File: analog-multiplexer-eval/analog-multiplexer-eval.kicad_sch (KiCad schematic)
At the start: 1 part, among them U1 4051

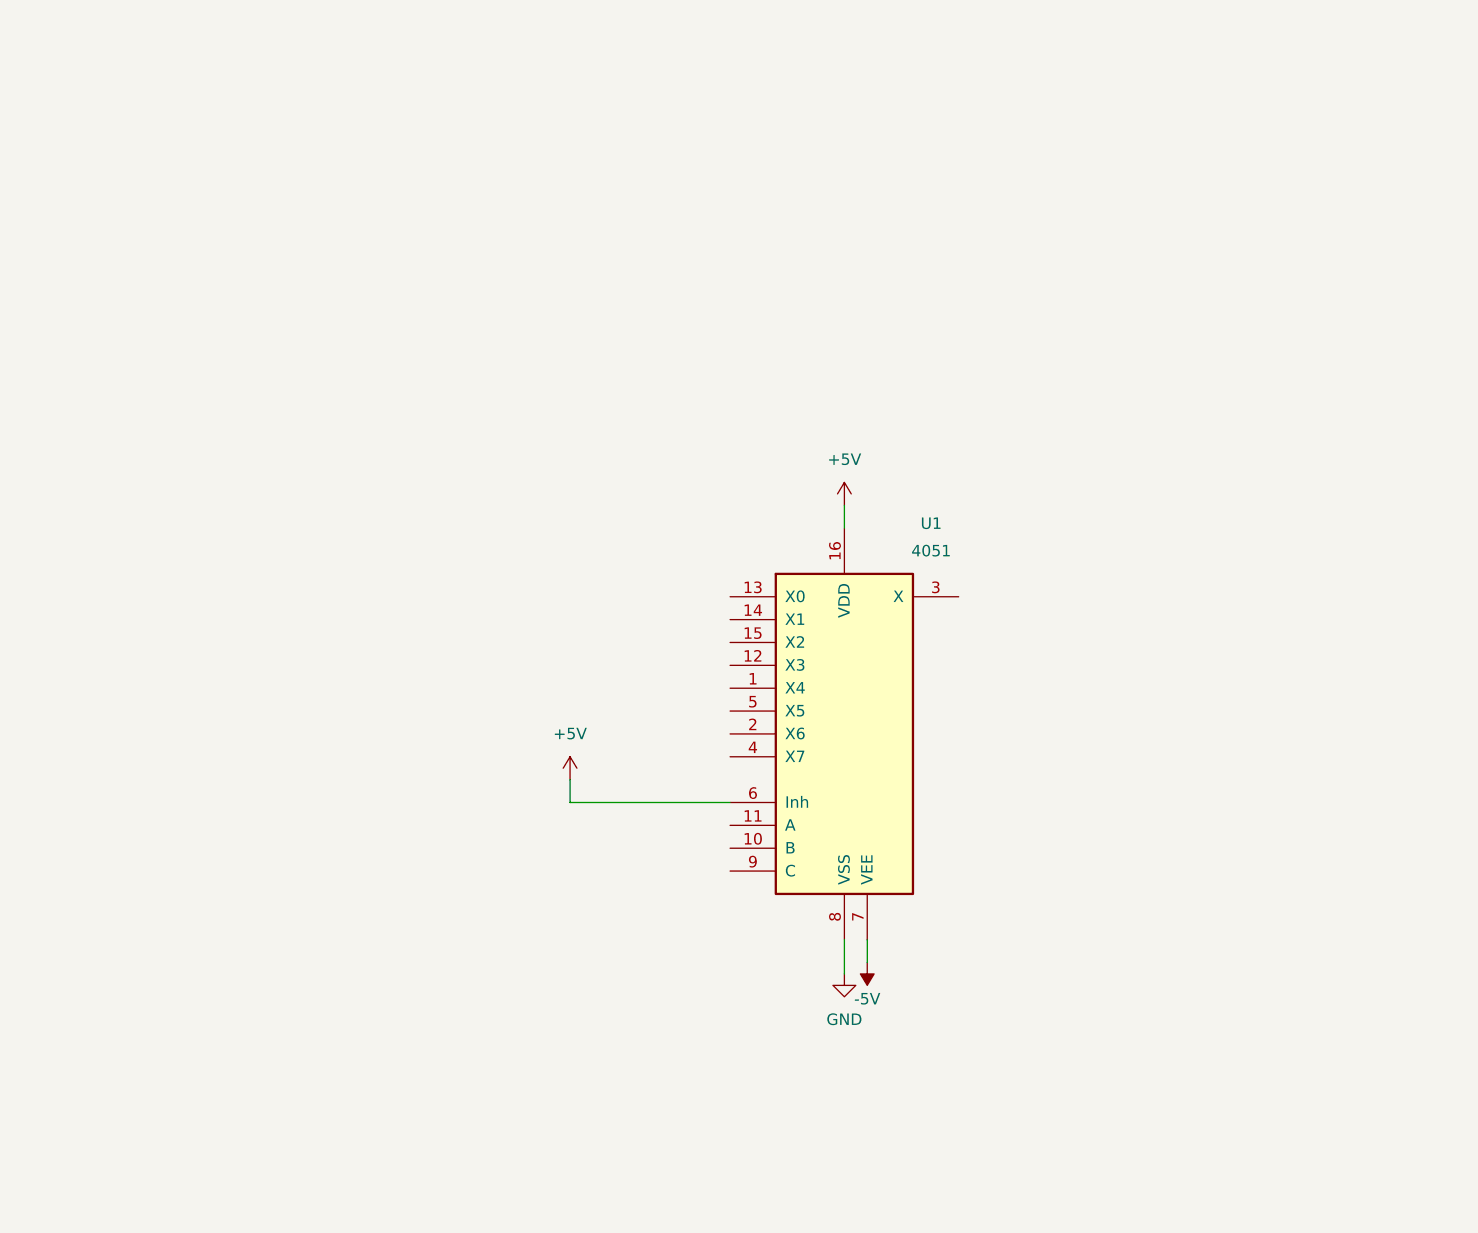
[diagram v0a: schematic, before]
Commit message: dvgsdgsd
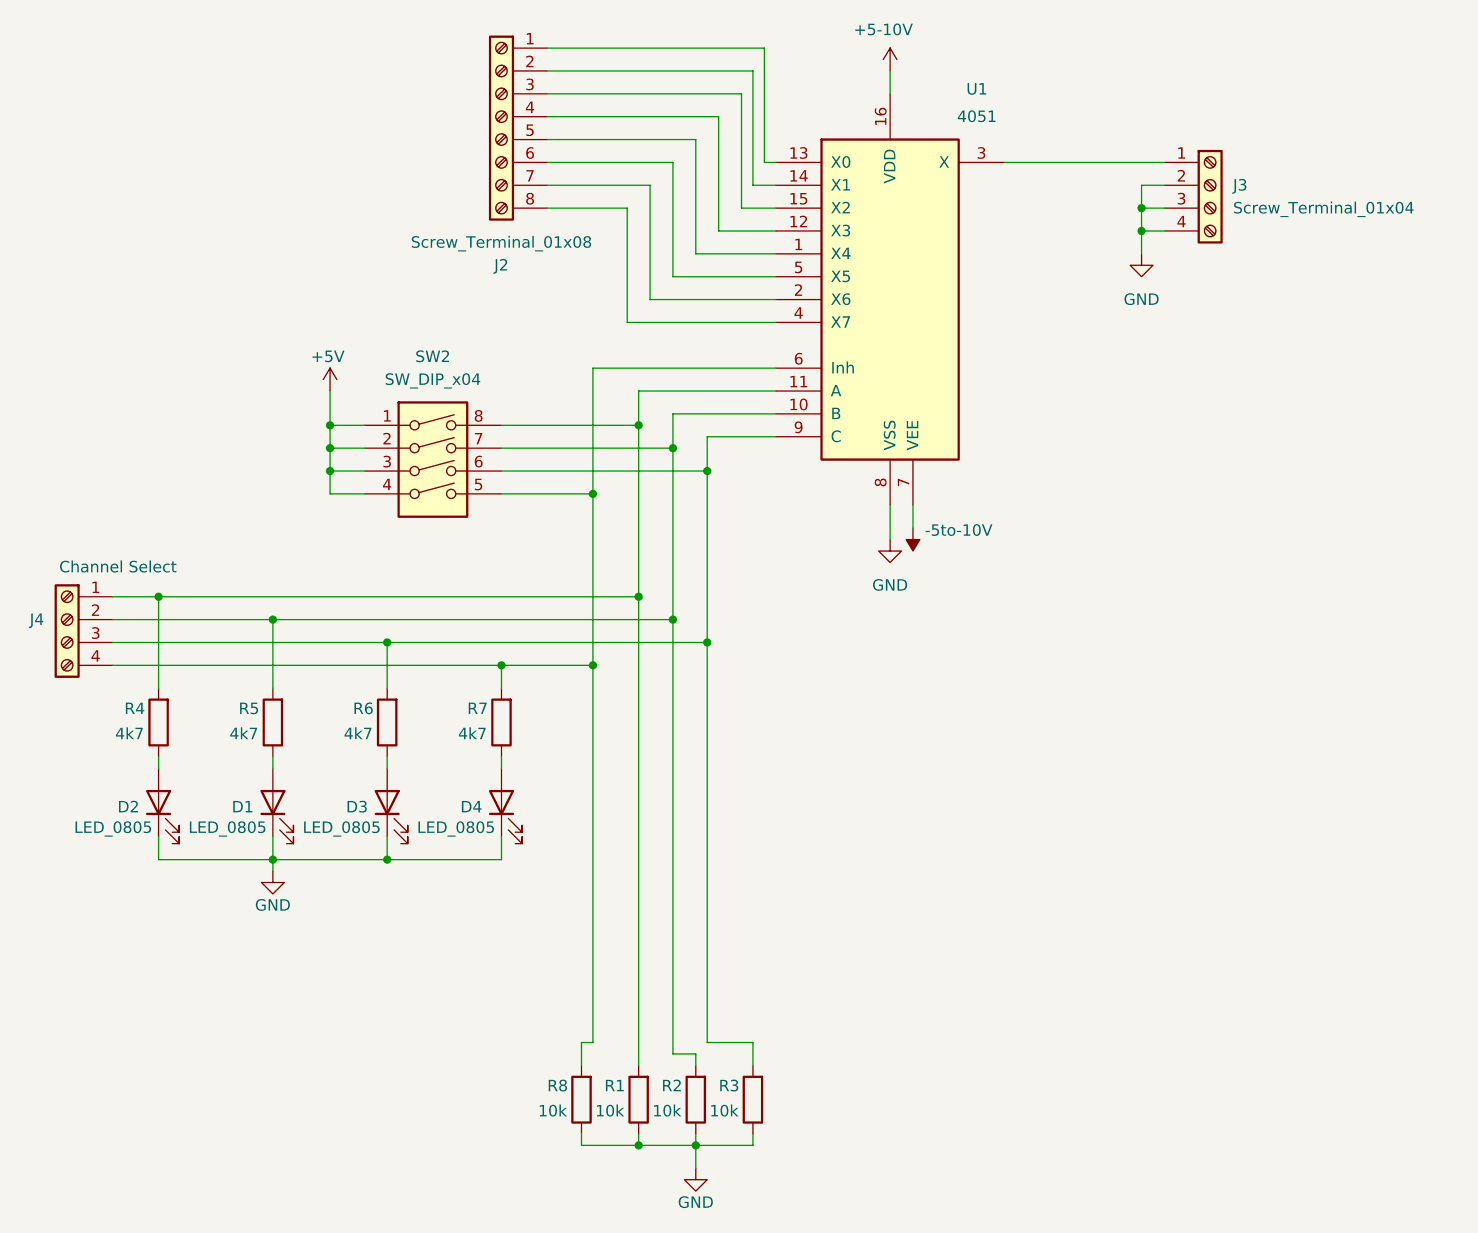
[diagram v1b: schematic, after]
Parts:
- added D1, D2, D3, D4: LED_0805, 000_Diodes_Immo:LED_0805_2012_Kawaii, symbol 000_Diodes_Immo:LED_0805_kawaii
- added J2: Screw_Terminal_01x08, symbol Connector:Screw_Terminal_01x08
- added J3: Screw_Terminal_01x04, symbol Connector:Screw_Terminal_01x04
- added J4: Channel Select, symbol Connector:Screw_Terminal_01x04
- added R1, R2, R3, R8: 10k, Resistor_SMD:R_0805_2012Metric_Pad1.20x1.40mm_HandSolder, symbol 000_Resistors_Immo:10k
- added R4, R5, R6, R7: 4k7, Resistor_SMD:R_0805_2012Metric_Pad1.20x1.40mm_HandSolder, symbol 000_Resistors_Immo:10k
- added SW2: SW_DIP_x04, symbol Switch:SW_DIP_x04
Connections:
- net +5V: now also SW2.1, SW2.2, SW2.3, SW2.4; no longer U1.16 (VDD), U1.6 (Inh)
- net GND: now also D1.1 (K), D2.1 (K), D3.1 (K), D4.1 (K), J3.2 (Pin_2), J3.3 (Pin_3), J3.4 (Pin_4), R1.1, R2.1, R3.1, R8.1
- net at U1.1 (X4): now also J2.5 (Pin_5)
- net at U1.10 (B): now also J4.2 (Pin_2), R2.2, R5.2, SW2.7
- net at U1.11 (A): now also J4.1 (Pin_1), R1.2, R4.2, SW2.8
- net at U1.12 (X3): now also J2.4 (Pin_4)
- net at U1.13 (X0): now also J2.1 (Pin_1)
- net at U1.14 (X1): now also J2.2 (Pin_2)
- net at U1.15 (X2): now also J2.3 (Pin_3)
- net at U1.2 (X6): now also J2.7 (Pin_7)
- net at U1.3 (X): now also J3.1 (Pin_1)
- net at U1.4 (X7): now also J2.8 (Pin_8)
- net at U1.5 (X5): now also J2.6 (Pin_6)
- net at U1.9 (C): now also J4.3 (Pin_3), R3.2, R6.2, SW2.6
- net -5V renamed -5to-10V
- new net: D3.2 (A), R6.1
- new net: J4.4 (Pin_4), R7.2, R8.2, SW2.5, U1.6 (Inh)
- new net: D4.2 (A), R7.1
- new net: D1.2 (A), R5.1
- new net: D2.2 (A), R4.1
- new net +5-10V: U1.16 (VDD)
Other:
- moved on the sheet: U1
